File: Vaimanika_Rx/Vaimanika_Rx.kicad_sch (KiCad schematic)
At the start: 1 part, among them U1 LR1121IMLTRT

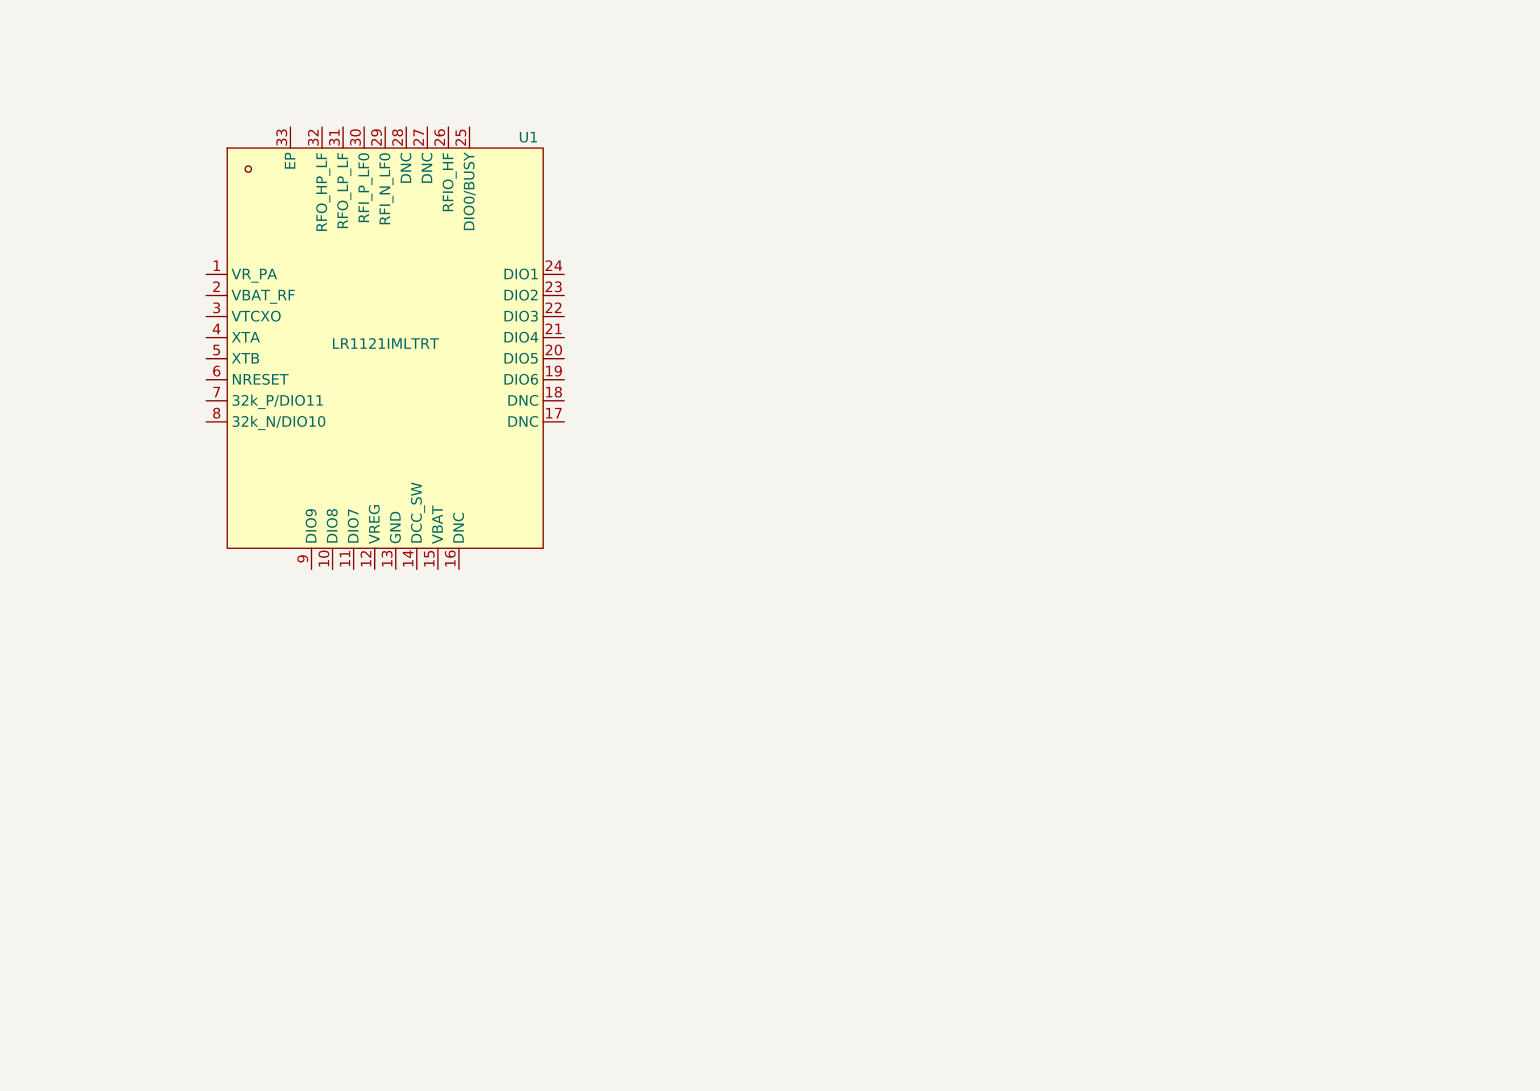
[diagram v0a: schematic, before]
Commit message: 12-05-2026
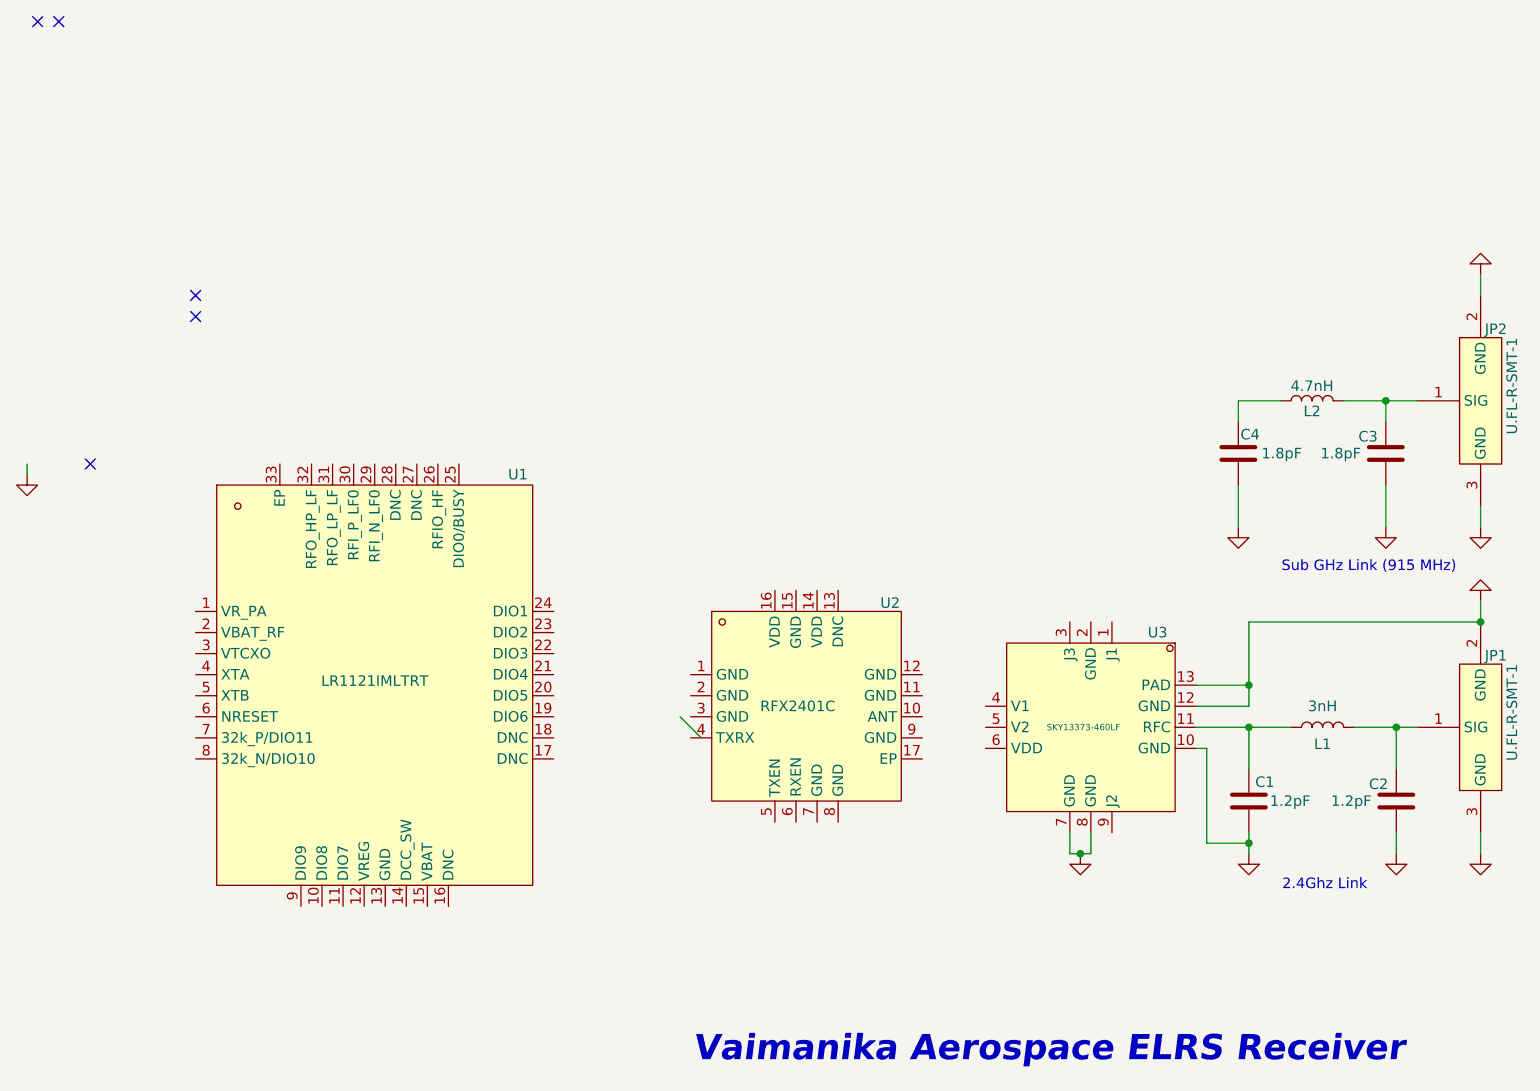
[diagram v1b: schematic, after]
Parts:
- added C1, C2: 1.2pF, Capacitor_SMD:C_0402_1005Metric, symbol Device:C
- added C3, C4: 1.8pF, Capacitor_SMD:C_0402_1005Metric, symbol Device:C
- added JP1, JP2: U.FL-R-SMT-1, New_Library:RF-SMD_FRF05002-JSS103M, symbol New_Library:U.FL-R-SMT-1
- added L1: 3nH, Inductor_SMD:L_0402_1005Metric, symbol Device:L
- added L2: 4.7nH, Inductor_SMD:L_0402_1005Metric, symbol Device:L
- added U2: RFX2401C, easyeda2kicad:QFN-16_L3.0-W3.0-P0.50-BL-EP1.7, symbol New_Library:RFX2401C
- added U3: SKY13373-460LF, easyeda2kicad:QFN-12_L2.0-W2.0-P0.50-BL-EP, symbol New_Library:SKY13373-460LF
- U1: footprint easyeda2kicad:QFN-32_L5.0-W5.0-P0.50-BL-EP3.7 -> New_Library:QFN-32_L5.0-W5.0-P0.50-BL-EP3.7; LCSC (none) -> C7498014; LCSC Part C7498014 -> (none)
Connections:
- new net: C2.1, JP1.1 (SIG), L1.2
- new net: C4.1, L2.1
- new net: C1.1, L1.1, U3.11 (RFC)
- new net: C3.1, JP2.1 (SIG), L2.2
- new net GND: C1.2, C2.2, C3.2, C4.2, JP1.2 (GND), JP1.3 (GND), JP2.2 (GND), JP2.3 (GND), U3.10 (GND), U3.12 (GND), U3.13 (PAD), U3.7 (GND), U3.8 (GND)
- no-connect marks 0 -> 5
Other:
- note added: "2.4Ghz Link"
- note added: "Sub GHz Link (915 MHz)"
- note added: "Vaimanika Aerospace ELRS Receiver"
- title: (none) -> ELRS Receiver 
- moved on the sheet: U1

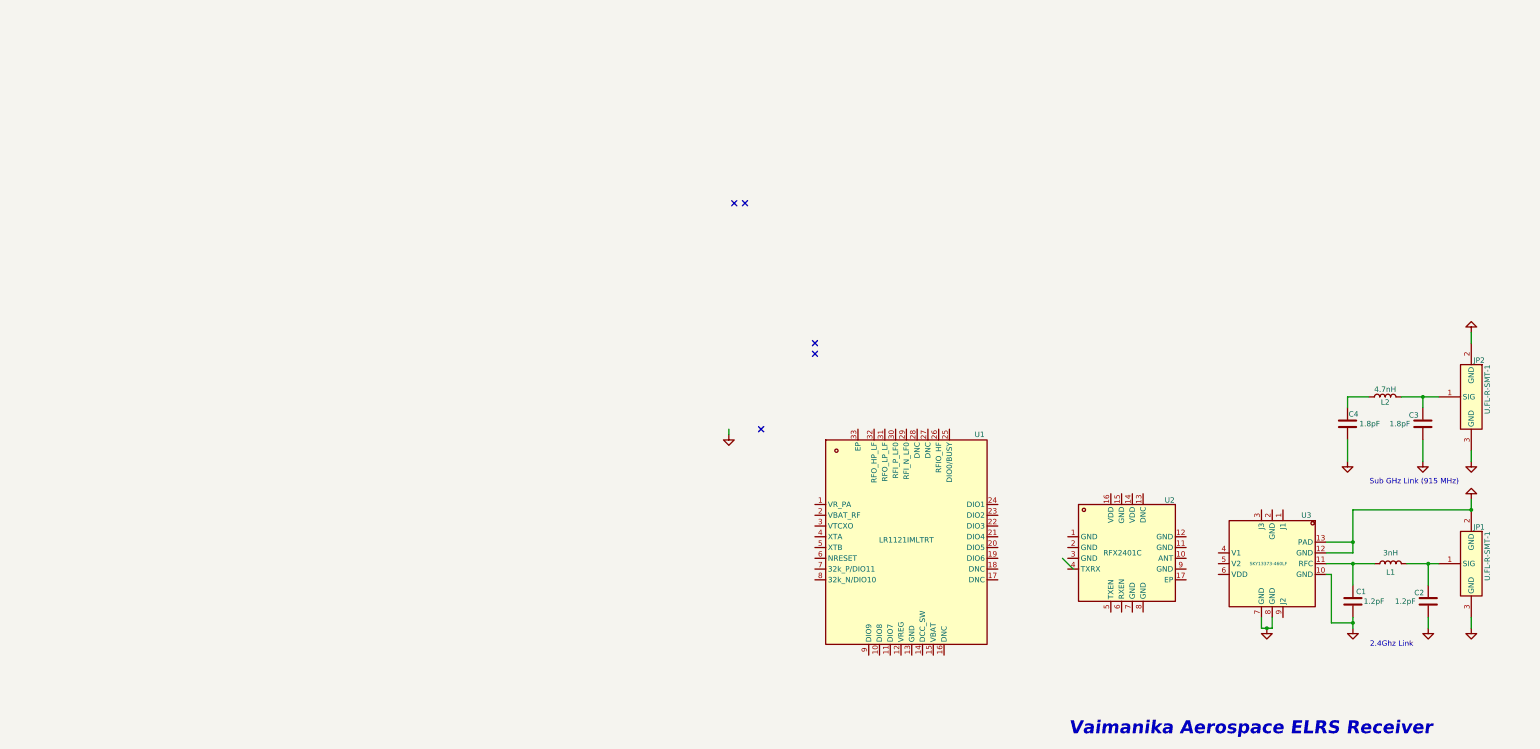
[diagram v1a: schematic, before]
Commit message: 14-05-2026
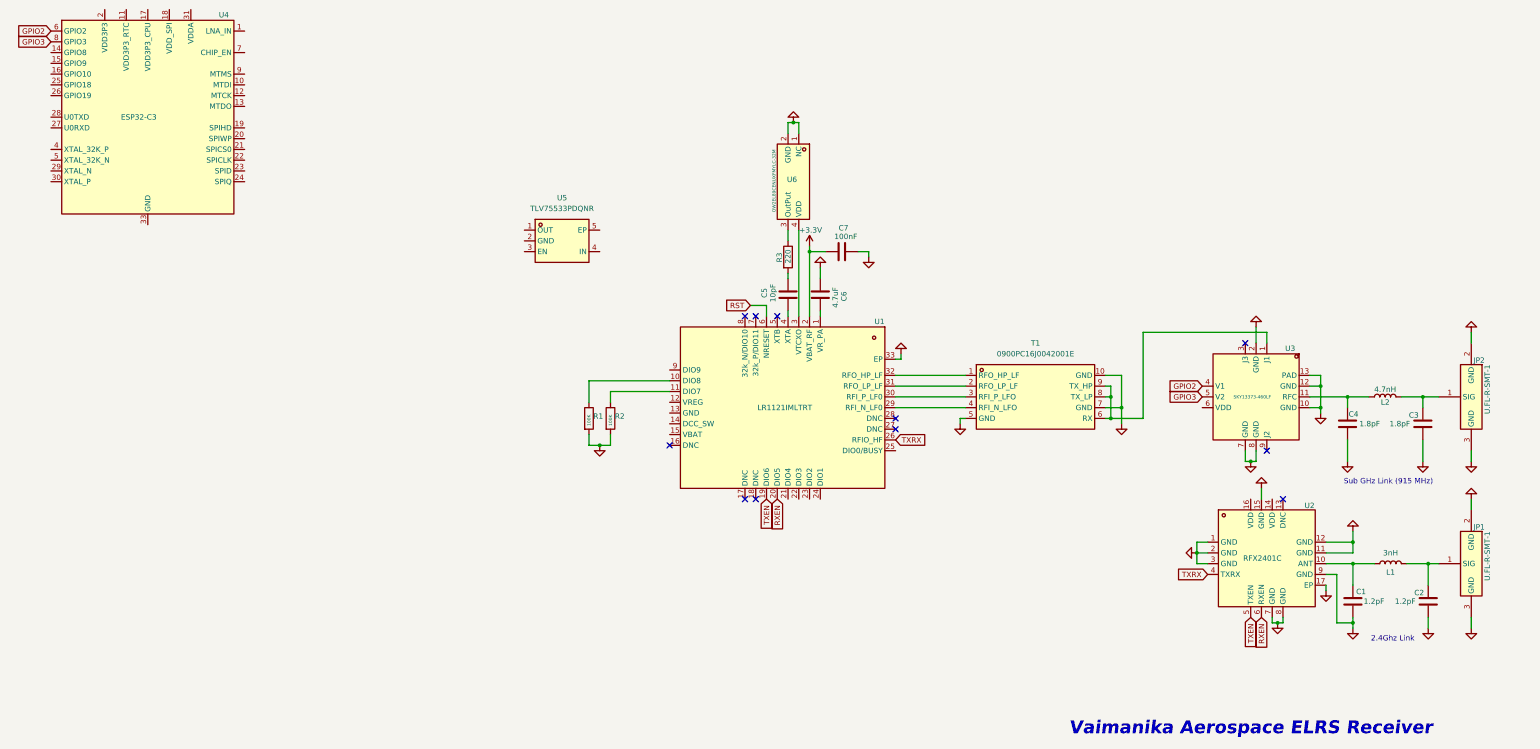
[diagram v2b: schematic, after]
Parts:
- added C5: 10pF, Capacitor_SMD:C_0402_1005Metric, symbol Device:C
- added C6: 4.7uF, Capacitor_SMD:C_0402_1005Metric, symbol Device:C
- added C7: 100nF, Capacitor_SMD:C_0402_1005Metric, symbol Device:C
- added R1, R2: 100K, Resistor_SMD:R_0402_1005Metric, symbol Device:R
- added R3: 220, Resistor_SMD:R_0402_1005Metric, symbol Device:R
- added T1: 0900PC16J0042001E, easyeda2kicad:FILTER-SMD_10P-L2.0-W1.6-BL, symbol New_Library:0900PC16J0042001E
- added U4: ESP32-C3, Package_DFN_QFN:QFN-32-1EP_5x5mm_P0.5mm_EP3.7x3.7mm, symbol MCU_Espressif:ESP32-C3
- added U5: TLV75533PDQNR, easyeda2kicad:X2SON-4_L1.0-W1.0-P0.65-TL-EP, symbol New_Library:TLV75533PDQNR
- added U6: OW2EL89CENUXFMYLC-32M, easyeda2kicad:OSC-SMD_4P-L3.2-W2.5-BL, symbol New_Library:OW2EL89CENUXFMYLC-32M
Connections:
- net GND: now also U1.33 (EP), U2.1 (GND), U2.11 (GND), U2.12 (GND), U2.15 (GND), U2.17 (EP), U2.2 (GND), U2.3 (GND), U2.7 (GND), U2.8 (GND), U2.9 (GND), U3.2 (GND), C6.2, C7.1, R1.2, R2.2, T1.10 (GND), T1.5 (GND), T1.7 (GND), U6.1 (NC), U6.2 (GND)
- net at C4.1, L2.1: now also U3.11 (RFC)
- net at U3.1 (J1): now also T1.6 (RX), T1.8 (TX_LP), T1.9 (TX_HP)
- net at C1.1, L1.1: now also U2.10 (ANT); no longer U3.11 (RFC)
- net GPIO2: now reaches U3.4 (V1)
- net GPIO2: now also U4.6 (GPIO2)
- net GPIO3: now reaches U3.5 (V2)
- net GPIO3: now also U4.8 (GPIO3)
- net at U1.1 (VR_PA): now also C6.1
- net at U1.10 (DIO8): now also R1.1
- net at U1.11 (DIO7): now also R2.1
- net TXEN: now reaches U1.19 (DIO6)
- net TXEN: now also U2.5 (TXEN)
- net +3.3V: now reaches U1.2 (VBAT_RF)
- net +3.3V: now also C7.2
- net RXEN: now reaches U1.20 (DIO5)
- net RXEN: now also U2.6 (RXEN)
- net TXRX: now reaches U1.26 (RFIO_HF)
- net TXRX: now also U2.4 (TXRX)
- net at U1.29 (RFI_N_LF0): now also T1.4 (RFI_N_LFO)
- net at U1.3 (VTCXO): now also U6.4 (VDD)
- net at U1.30 (RFI_P_LF0): now also T1.3 (RFI_P_LFO)
- net at U1.31 (RFO_LP_LF): now also T1.2 (RFO_LP_LF)
- net at U1.32 (RFO_HP_LF): now also T1.1 (RFO_HP_LF)
- net at U1.4 (XTA): now also C5.2
- net RST: now reaches U1.6 (NRESET)
- new net: R3.1, U6.3 (OutPut)
- new net: C5.1, R3.2
- new net: U4.2 (VDD3P3), U4.3 (VDD3P3)
- new net: U4.31 (VDDA), U4.32 (VDDA)
- no-connect marks 5 -> 11
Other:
- moved on the sheet: U1, U2, U3

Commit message: 18-05-2026
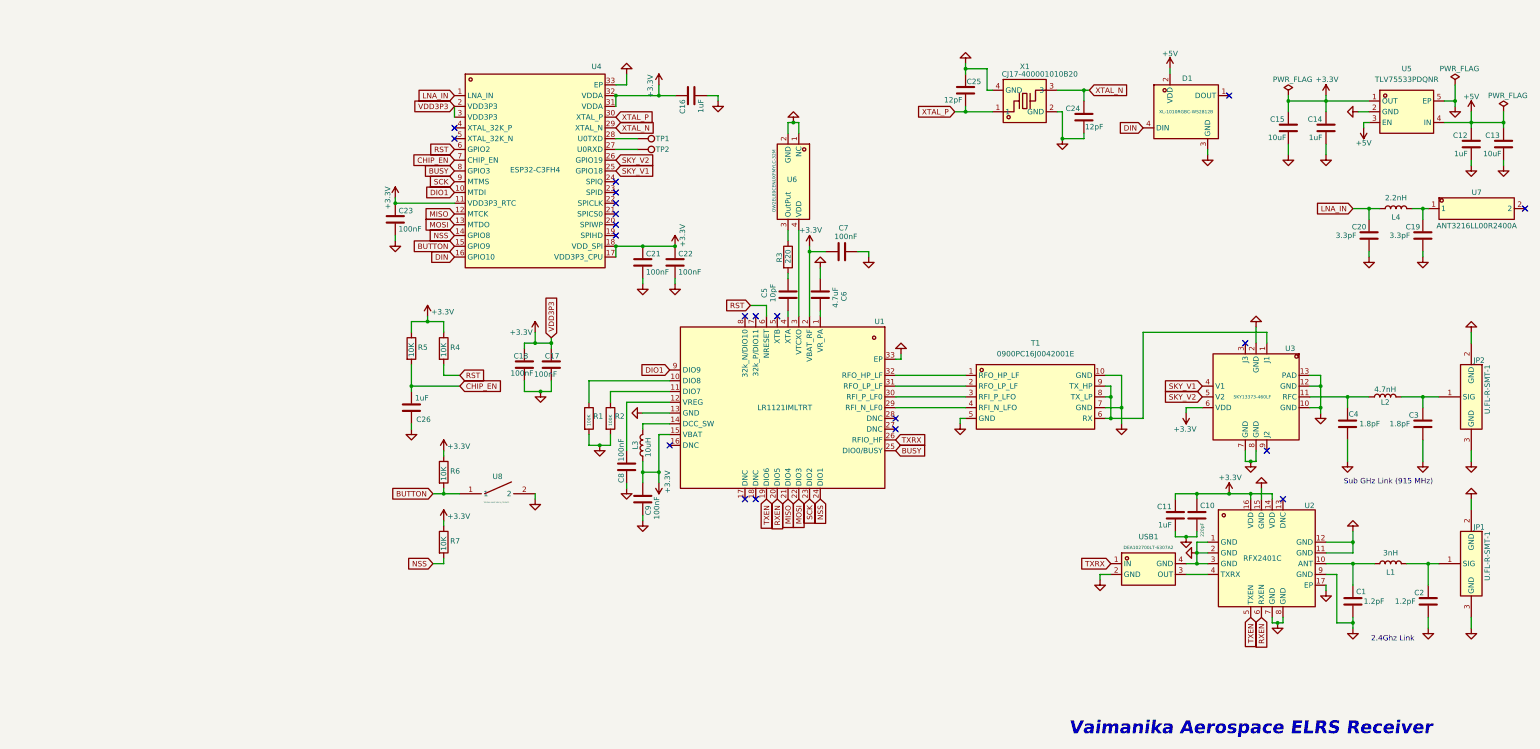
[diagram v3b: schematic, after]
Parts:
- removed U4: ESP32-C3, Package_DFN_QFN:QFN-32-1EP_5x5mm_P0.5mm_EP3.7x3.7mm, symbol MCU_Espressif:ESP32-C3
- added C10: 220pF, Capacitor_SMD:C_0402_1005Metric, symbol Device:C
- added C11, C12, C14, C16, C26: 1uF, Capacitor_SMD:C_0402_1005Metric, symbol Device:C
- added C13, C15: 10uF, Capacitor_SMD:C_0402_1005Metric, symbol Device:C
- added C17, C18, C21, C22, C23, C8, C9: 100nF, Capacitor_SMD:C_0402_1005Metric, symbol Device:C
- added C19, C20: 3.3pF, Capacitor_SMD:C_0402_1005Metric, symbol Device:C
- added C24, C25: 12pF, Capacitor_SMD:C_0402_1005Metric, symbol Device:C
- added D1: XL-1010RGBC-WS2812B, New_Library:LED-SMD_4P-L1.0-W1.0-TL_XL-1010RGBC-WS2812B, symbol New_Library:XL-1010RGBC-WS2812B
- added L3: 10uH, Inductor_SMD:L_0603_1608Metric, symbol Device:L
- added L4: 2.2nH, Inductor_SMD:L_0402_1005Metric, symbol Device:L
- added R4, R5, R6, R7: 10K, Resistor_SMD:R_0402_1005Metric, symbol Device:R
- added TP1, TP2: TestPoint, Connector_Wire:SolderWirePad_1x01_SMD_1x2mm, symbol Connector:TestPoint
- added U4: ESP32-C3FH4, New_Library:QFN-32_L5.0-W5.0-P0.50-BL-EP3.7, symbol New_Library:ESP32-C3FH4
- added U7: ANT3216LL00R2400A, New_Library:ANT-SMD_L3.2-W1.6, symbol New_Library:ANT3216LL00R2400A
- added U8: TS2306A 240GF MSM 9_C2976675, New_Library:SW-SMD_4P-L3.0-W2.0-P0.85-LS3.5, symbol New_Library:TS2306A240GFMSM9_C2976675
- added USB1: DEA102700LT-6307A2, New_Library:FILTER-SMD_4P-L1.0-W0.5-L_DEA102700LT-XXX, symbol New_Library:DEA102700LT-6307A2
- added X1: CJ17-400001010B20, easyeda2kicad:CRYSTAL-SMD_4P-L1.6-W1.2-BL, symbol New_Library:CJ17-400001010B20
- T1: footprint easyeda2kicad:FILTER-SMD_10P-L2.0-W1.6-BL -> New_Library:FILTER-SMD_10P-L2.0-W1.6-BL; LCSC (none) -> C19842466; LCSC Part C19842466 -> (none)
- U2: footprint easyeda2kicad:QFN-16_L3.0-W3.0-P0.50-BL-EP1.7 -> New_Library:QFN-16_L3.0-W3.0-P0.50-BL-EP1.7
- U3: footprint easyeda2kicad:QFN-12_L2.0-W2.0-P0.50-BL-EP -> New_Library:QFN-12_L2.0-W2.0-P0.50-BL-EP
- U5: footprint easyeda2kicad:X2SON-4_L1.0-W1.0-P0.65-TL-EP -> New_Library:X2SON-4_L1.0-W1.0-P0.65-TL-EP
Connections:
- net +3.3V: now also U1.15 (VBAT), U2.14 (VDD), U2.16 (VDD), U3.6 (VDD), U5.1 (OUT), C10.1, C11.1, C14.1, C15.1, C16.1, C17.1, C18.1, C21.1, C22.1, C23.1, C9.1, L3.1, R4.1, R5.1, R6.1, R7.1, U4.11 (VDD3P3_RTC), U4.17 (VDD3P3_CPU), U4.18 (VDD_SPI), U4.2 (VDD3P3), U4.3 (VDD3P3), U4.31 (VDDA), U4.32 (VDDA)
- net GND: now also U1.13 (GND), U5.2 (GND), U5.5 (EP), C10.2, C11.2, C12.2, C13.2, C14.2, C15.2, C16.2, C17.2, C18.2, C19.2, C20.2, C21.2, C22.2, C23.2, C24.2, C25.1, C26.1, C8.2, C9.2, D1.3 (GND), U4.33 (EP), U8.2, USB1.2 (GND), USB1.4 (GND), X1.2 (GND), X1.4 (GND)
- net RST: now also R4.2, U4.6 (GPIO2)
- net TXRX: now also USB1.1 (IN); no longer U2.4 (TXRX)
- net +5V: now reaches U5.3 (EN)
- net +5V: now also U5.4 (IN), C12.1, C13.1, D1.2 (VDD)
- net at U1.12 (VREG): now also C8.1
- net at U1.14 (DCC_SW): now also L3.2
- net MISO: now reaches U1.21 (DIO4)
- net MISO: now also U4.12 (MTCK)
- net MOSI: now reaches U1.22 (DIO3)
- net MOSI: now also U4.13 (MTDO)
- net SCK: now reaches U1.23 (DIO2)
- net SCK: now also U4.9 (MTMS)
- net NSS: now reaches U1.24 (DIO1)
- net NSS: now also R7.2, U4.14 (GPIO8)
- net BUSY: now reaches U1.25 (DIO0/BUSY)
- net BUSY: now also U4.8 (GPIO3)
- net DIO1: now reaches U1.9 (DIO9)
- net DIO1: now also U4.10 (MTDI)
- net GPIO2 renamed SKY_V1
- net SKY_V1: now also U4.25 (GPIO18)
- net GPIO3 renamed SKY_V2
- net SKY_V2: now also U4.26 (GPIO19)
- new net: U2.4 (TXRX), USB1.3 (OUT)
- new net: TP2.1, U4.27 (U0RXD)
- new net: C19.1, L4.2, U7.1
- new net: TP1.1, U4.28 (U0TXD)
- new net BUTTON: R6.2, U4.15 (GPIO9), U8.1
- new net CHIP_EN: C26.2, R5.2, U4.7 (CHIP_EN)
- new net DIN: D1.4 (DIN), U4.16 (GPIO10)
- new net LNA_IN: C20.1, L4.1, U4.1 (LNA_IN)
- new net XTAL_N: C24.1, U4.29 (XTAL_N), X1.3
- new net XTAL_P: C25.2, U4.30 (XTAL_P), X1.1
- no-connect marks 11 -> 21
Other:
- moved on the sheet: U5
